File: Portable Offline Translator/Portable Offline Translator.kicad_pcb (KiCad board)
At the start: 2 copper layers, 121.4 x 144.4 mm, 59 parts, among them IC301 STM32F407IET6, J201 Conn_01x08_Male, J301 Conn_02x03_Odd_Even, SW301 SW_Push, SW303 SW_Push, SW305 SW_Push, SW306 SW_Push, U202 MAX98357AETE_T, U401 LM317_SOT-223, U402 LM317_SOT-223, Y301 Crystal

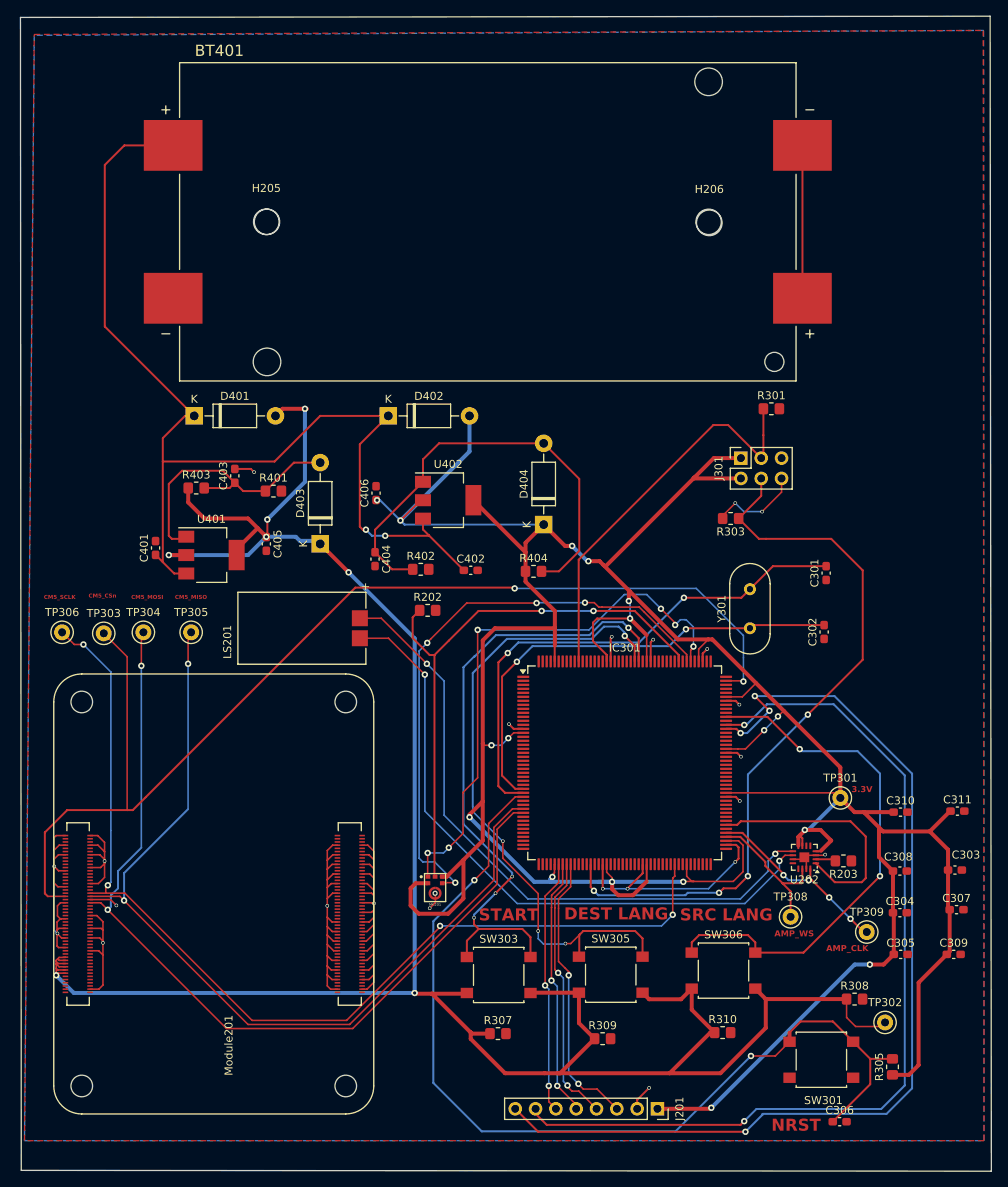
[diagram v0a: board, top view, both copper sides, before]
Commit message: main PCB v1 done
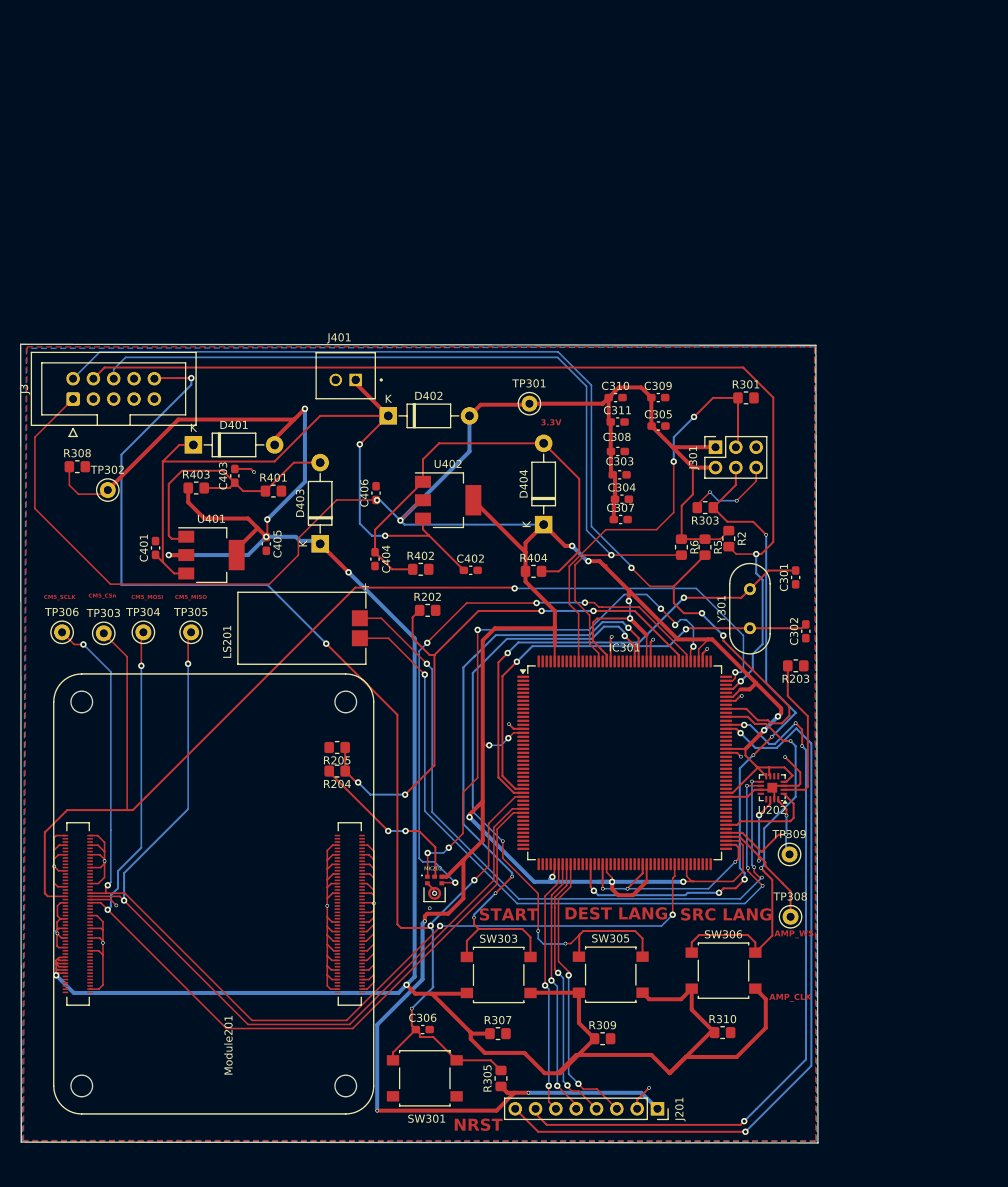
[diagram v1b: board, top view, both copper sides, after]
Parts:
- removed BT401: 1048P, 1048P(16850 Dual Bat Holder:BAT_1048P
- removed H205, H206: MountingHole, MountingHole:MountingHole_3.2mm_M3
- removed MK201: ICS-43434, ICS_43434(MIC):MIC_ICS-43434
- added J3: Conn_ARM_JTAG_SWD_10, Connector_IDC:IDC-Header_2x05_P2.54mm_Vertical, F.Cu at (84.3, 61.8)
- added J401: B2B-XH-A, Battery Connector(JST-XH):JST_B2B-XH-A, F.Cu at (118.4, 58.9)
- added MK202: SPH0645LM4H-B, SPH0645LM4H-B(Microphone):MIC_SPH0645LM4H-B, F.Cu at (129.5, 123.6)
- added R2: 100k, Resistor_SMD:R_0805_2012Metric_Pad1.20x1.40mm_HandSolder, F.Cu at (166.3, 79.2)
- added R204: 51, Resistor_SMD:R_0805_2012Metric_Pad1.20x1.40mm_HandSolder, F.Cu at (117.3, 108.3)
- added R205: 100k, Resistor_SMD:R_0805_2012Metric_Pad1.20x1.40mm_HandSolder, F.Cu at (117.3, 105.3)
- added R5: 100k, Resistor_SMD:R_0805_2012Metric_Pad1.20x1.40mm_HandSolder, F.Cu at (163.3, 80.3)
- added R6: 100k, Resistor_SMD:R_0805_2012Metric_Pad1.20x1.40mm_HandSolder, F.Cu at (160.3, 80.3)
- moved R308 117.8 mm to (84.8, 70.2)
- moved TP302 117.8 mm to (88.6, 73.2)
- moved C309 78.8 mm to (157.5, 61.6)
- moved C305 72.6 mm to (157.5, 65.2)
- moved C308 67.2 mm to (152.4, 68.3)
- moved C311 64.6 mm to (152.4, 64.6)
- moved C307 64.4 mm to (152.8, 76.8)
- moved C310 62.9 mm to (152.1, 61.6)
- moved TP301 62.8 mm to (141.4, 62.4)
- moved C304 62.3 mm to (152.9, 74.3)
- moved C303 60.7 mm to (152.6, 71.2)
- moved C306 53.4 mm to (128.0, 140.6)
- moved SW301 49.6 mm to (128.3, 146.7)
- moved R305 49.0 mm to (137.8, 146.7)
- moved R203 25.1 mm to (174.6, 95.1)
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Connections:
- IC301 pad 124: unconnected-(IC301-PA13-Pad124) -> /MCU/JTMS/SWDIO
- IC301 pad 129: unconnected-(IC301-PH14-Pad129) -> /MCU/JTCK/SWCLK
- IC301 pad 161: unconnected-(IC301-PB3-Pad161) -> /MCU/JTDO/TRACESWO
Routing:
- net /MCU/JTMS/SWDIO: track 0.00 -> 137.1 mm, vias 0 -> 3
- net /MCU/JTCK/SWCLK: track 0.00 -> 131.5 mm, vias 0 -> 2
- net /MCU/JTDO/TRACESWO: track 0.00 -> 111.9 mm, vias 0 -> 1
- net /PowerSS/REG_IN: track 134.5 -> 91.6 mm
- net /MCU/NRST: track 119.0 -> 160.0 mm, vias 2 -> 5
- net +3.3V: track 461.0 -> 497.7 mm
- net /IO Circuits/LCD_RST: track 125.5 -> 95.3 mm, vias 4 -> 2
- net /IO Circuits/LCD_Data/Command: track 115.2 -> 92.0 mm, vias 2 -> 4
- net Net-(MK202-DATA_OUT): track 0.00 -> 21.0 mm, vias 0 -> 2
- net +5V: track 300.0 -> 320.7 mm
- net Net-(BT401-PadN1): track 19.1 -> 0.00 mm
- net /IO Circuits/AMP_I2S2_SD: track 31.1 -> 12.3 mm
- net Net-(U202-GAIN_SLOT): track 2.53 -> 19.3 mm
- net Net-(IC301-PA11): track 65.8 -> 50.5 mm
- net /IO Circuits/OUTN: track 81.0 -> 90.1 mm, vias 2 -> 4
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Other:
- board size 121.4 x 144.4 mm -> 99.7 x 99.8 mm
